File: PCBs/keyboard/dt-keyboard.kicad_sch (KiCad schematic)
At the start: 87 parts

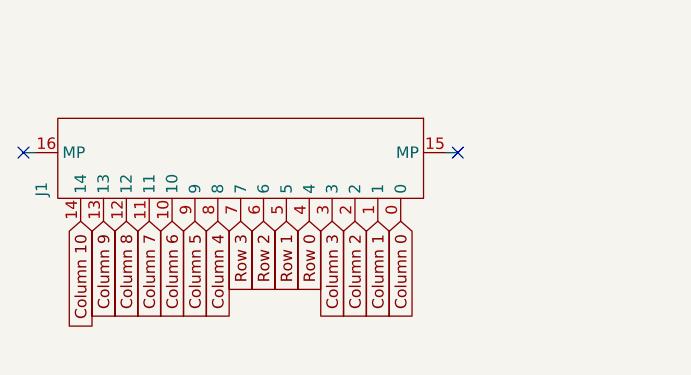
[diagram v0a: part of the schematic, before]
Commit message: Layouting + Deep Sleep Tests
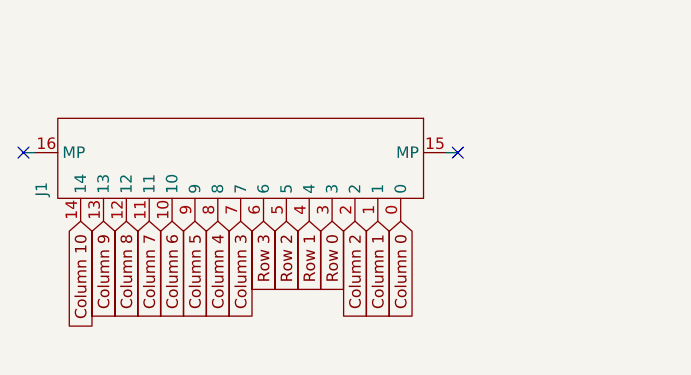
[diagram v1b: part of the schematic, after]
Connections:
- net Column 3: now also J1.7; no longer J1.3
- net Row 0: now also J1.3; no longer J1.4
- net Row 1: now also J1.4; no longer J1.5
- net Row 2: now also J1.5; no longer J1.6
- net Row 3: now also J1.6; no longer J1.7
